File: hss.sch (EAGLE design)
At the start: 11 parts, among them IC1 MEGA328P, Q1 BUZ71

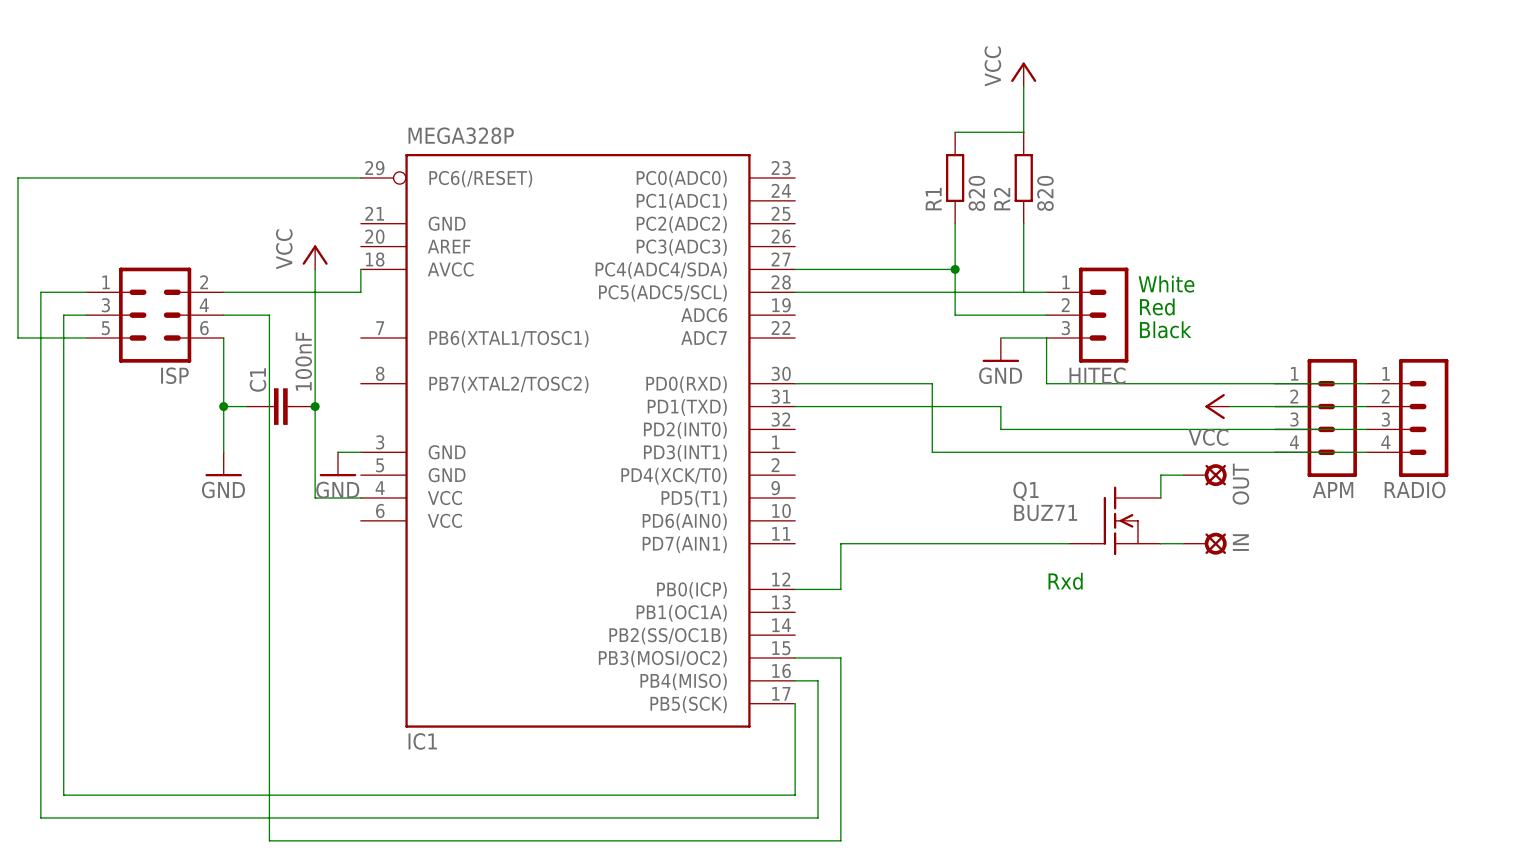
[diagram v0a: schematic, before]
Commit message: version 4 of the board
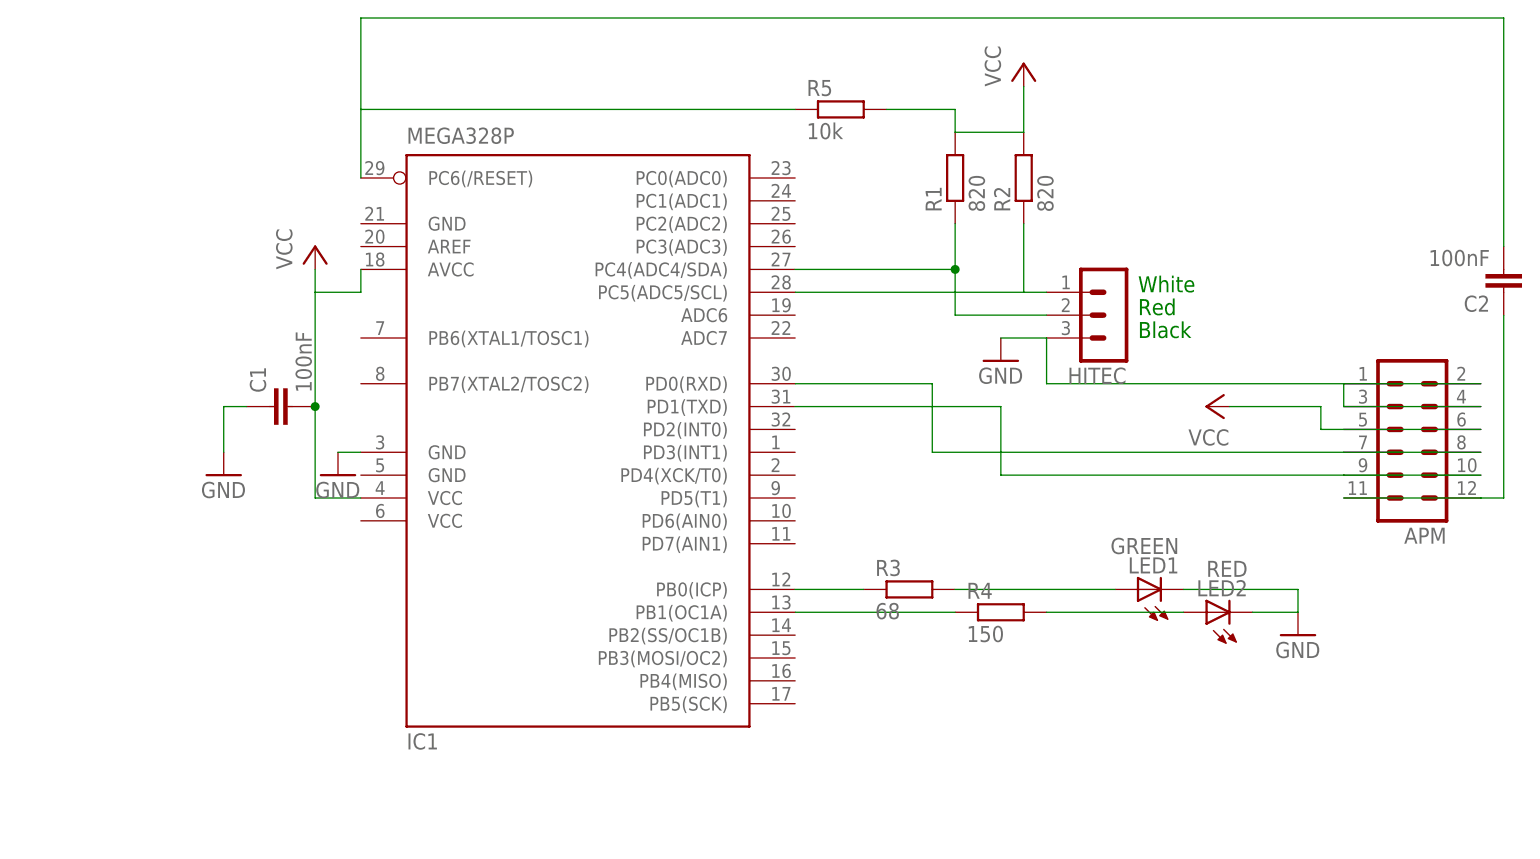
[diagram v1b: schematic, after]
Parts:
- removed IN, OUT: MCS08, solpad:MCS08
- removed ISP: (no value), con-lstb:MA03-2
- removed Q1: BUZ71, transistor-fet:BUZ71
- removed RADIO: (no value), con-lstb:MA04-1
- added C2: 100nF, resistor:C-EUC1206
- added LED1: GREEN, led:LEDSMT1206
- added LED2: RED, led:LEDSMT1206
- added R3: 68, resistor:R-EU_M1206
- added R4: 150, resistor:R-EU_M1206
- added R5: 10k, resistor:R-EU_M1206
- APM: device con-lstb:MA04-1 -> con-lstb:MA06-2
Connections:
- removed net N$11: IN.MP, Q1.S
- net GND: now also APM.2, APM.3, APM.4, LED1.C, LED2.C; no longer ISP.6, RADIO.1
- net N$1: now also IC1.PB0(ICP), R3.1; no longer IC1.PC6(/RESET), ISP.5
- net N$10: now also APM.11, APM.12, C2.1; no longer IC1.PB0(ICP), Q1.G
- net N$14: now also APM.10, APM.9; no longer APM.3, RADIO.3
- net N$15: now also APM.7, APM.8; no longer APM.4, RADIO.4
- net N$5: now also C2.2, IC1.PC6(/RESET), R5.1; no longer OUT.MP, Q1.D
- net N$7: now also LED1.A, R3.2; no longer IC1.PB5(SCK), ISP.3
- net N$8: now also IC1.PB1(OC1A), R4.1; no longer IC1.PB4(MISO), ISP.1
- net N$9: now also LED2.A, R4.2; no longer IC1.PB3(MOSI/OC2), ISP.4
- net VCC: now also APM.5, APM.6, R5.2; no longer APM.2, ISP.2, RADIO.2
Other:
- note removed: "Rxd"
